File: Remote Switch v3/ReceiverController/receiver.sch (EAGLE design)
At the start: 40 parts, among them IC1 LNK304, IC2 MCP1703CB, IC3 STM8L101F2, J1 POWER_CONN_4, T1 BT136

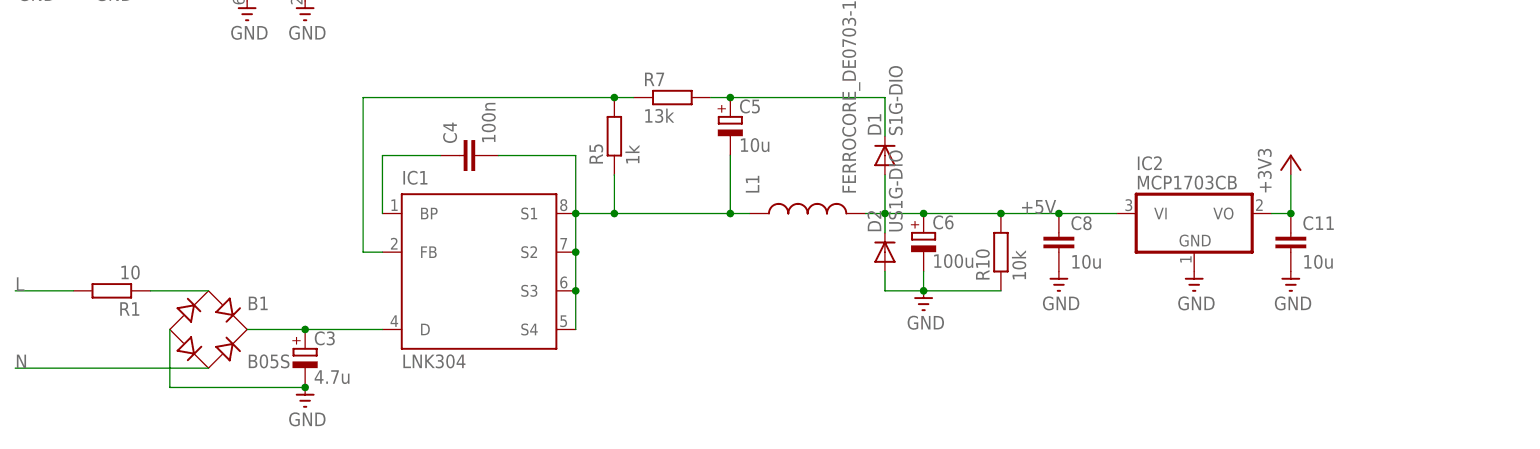
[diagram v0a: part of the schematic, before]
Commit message: PCB work
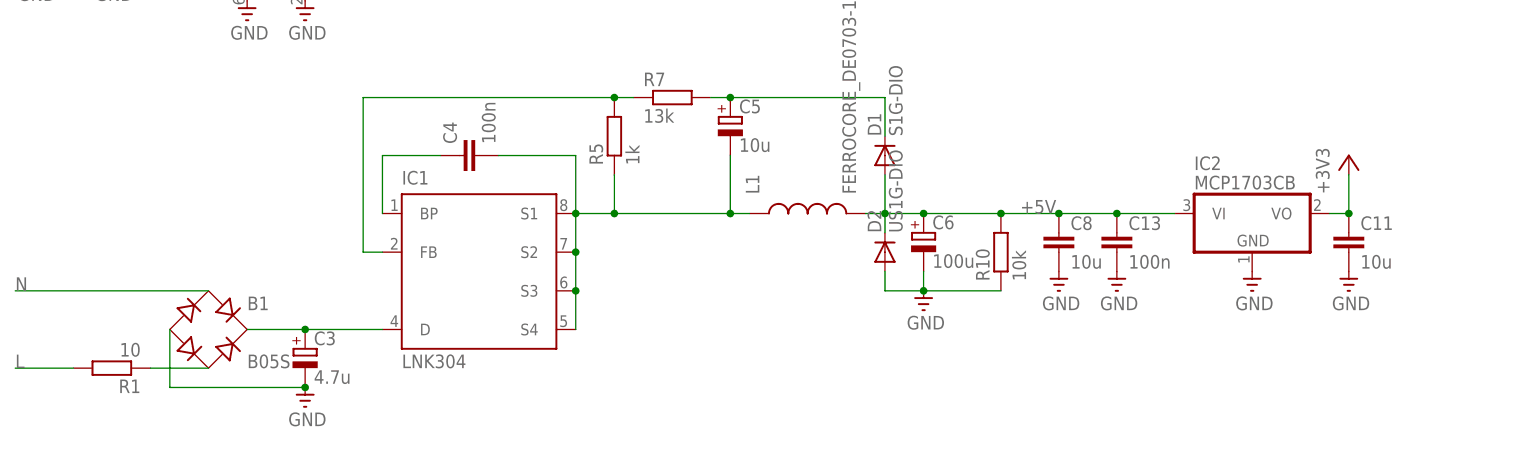
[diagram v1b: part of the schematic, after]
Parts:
- added C13: 100n, resistor:C-EUC0603K
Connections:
- removed net N$19: B1.AC1, R1.1
- new net N$10: B1.AC2, R1.1
- net +5V: now also C13.1
- net GND: now also C13.2
- net N: now also B1.AC1; no longer B1.AC2
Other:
- moved on the sheet: C11, IC2, R1
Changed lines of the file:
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@@
 <part name="GND1" library="supply" deviceset="GND" device=""/>
 <part name="R12" library="resistor" deviceset="R-EU_" device="R0603" value="47"/>
+<part name="C13" library="resistor" deviceset="C-EU" device="C0603K" value="100n"/>
+<part name="GND17" library="supply" deviceset="GND" device=""/>
 </parts>
 <sheets>
@@
 <instance part="GND15" gate="1" x="182.88" y="157.48" rot="R270"/>
 <instance part="LED1" gate="G$1" x="53.34" y="162.56" rot="R270"/>
-<instance part="R1" gate="G$1" x="25.4" y="43.18" rot="R180"/>
+<instance part="R1" gate="G$1" x="25.4" y="33.02" rot="R180"/>
 <instance part="C10" gate="G$1" x="160.02" y="142.24"/>
 <instance part="IC1" gate="G$1" x="73.66" y="45.72"/>
 <instance part="GND8" gate="1" x="132.08" y="40.64"/>
 <instance part="GND5" gate="1" x="50.8" y="27.94"/>
-<instance part="+3V34" gate="G$1" x="180.34" y="60.96"/>
+<instance part="+3V34" gate="G$1" x="187.96" y="60.96"/>
 <instance part="D2" gate="G$1" x="127" y="48.26" rot="R90"/>
 <instance part="L1" gate="G$1" x="116.84" y="53.34" rot="R90"/>
@@
 <instance part="R3" gate="G$1" x="63.5" y="134.62"/>
 <instance part="GND6" gate="1" x="66.04" y="121.92"/>
-<instance part="IC2" gate="G$1" x="167.64" y="53.34"/>
-<instance part="C11" gate="G$1" x="180.34" y="50.8"/>
-<instance part="GND14" gate="1" x="180.34" y="43.18"/>
+<instance part="IC2" gate="G$1" x="175.26" y="53.34"/>
+<instance part="C11" gate="G$1" x="187.96" y="50.8"/>
+<instance part="GND14" gate="1" x="187.96" y="43.18"/>
 <instance part="C8" gate="G$1" x="149.86" y="50.8"/>
-<instance part="GND13" gate="1" x="167.64" y="43.18"/>
+<instance part="GND13" gate="1" x="175.26" y="43.18"/>
 <instance part="GND10" gate="1" x="149.86" y="43.18"/>
 <instance part="RF1" gate="G$1" x="45.72" y="93.98"/>
@@
 <instance part="GND1" gate="1" x="15.24" y="83.82"/>
 <instance part="R12" gate="G$1" x="220.98" y="109.22"/>
+<instance part="C13" gate="G$1" x="157.48" y="50.8"/>
+<instance part="GND17" gate="1" x="157.48" y="43.18"/>
 </instances>
 <busses>
@@
 <junction x="238.76" y="134.62"/>
 <junction x="241.3" y="134.62"/>
+</segment>
+<segment>
+<pinref part="C13" gate="G$1" pin="2"/>
+<pinref part="GND17" gate="1" pin="GND"/>
 </segment>
 </net>
@@
 <pinref part="IC2" gate="G$1" pin="VO"/>
 <pinref part="C11" gate="G$1" pin="1"/>
-<wire x1="177.8" y1="53.34" x2="180.34" y2="53.34" width="0.1524" layer="91"/>
+<wire x1="185.42" y1="53.34" x2="187.96" y2="53.34" width="0.1524" layer="91"/>
 <pinref part="+3V34" gate="G$1" pin="+3V3"/>
-<wire x1="180.34" y1="53.34" x2="180.34" y2="58.42" width="0.1524" layer="91"/>
-<junction x="180.34" y="53.34"/>
+<wire x1="187.96" y1="53.34" x2="187.96" y2="58.42" width="0.1524" layer="91"/>
+<junction x="187.96" y="53.34"/>
 </segment>
 <segment>
@@
 </segment>
 <segment>
-<wire x1="38.1" y1="33.02" x2="12.7" y2="33.02" width="0.1524" layer="91"/>
-<label x="12.7" y="33.02" size="1.778" layer="95"/>
-<pinref part="B1" gate="G$1" pin="AC2"/>
+<pinref part="B1" gate="G$1" pin="AC1"/>
+<wire x1="38.1" y1="43.18" x2="12.7" y2="43.18" width="0.1524" layer="91"/>
+<label x="12.7" y="43.18" size="1.778" layer="95"/>
 </segment>
 </net>
@@
 </segment>
 </net>
-<net name="N$19" class="0">
-<segment>
-<pinref part="R1" gate="G$1" pin="1"/>
-<pinref part="B1" gate="G$1" pin="AC1"/>
-<wire x1="30.48" y1="43.18" x2="38.1" y2="43.18" width="0.1524" layer="91"/>
-</segment>
-</net>
 <net name="L" class="0">
 <segment>
@@
 <segment>
 <pinref part="R1" gate="G$1" pin="2"/>
-<wire x1="20.32" y1="43.18" x2="12.7" y2="43.18" width="0.1524" layer="91"/>
-<label x="12.7" y="43.18" size="1.778" layer="95"/>
+<wire x1="20.32" y1="33.02" x2="12.7" y2="33.02" width="0.1524" layer="91"/>
+<label x="12.7" y="33.02" size="1.778" layer="95"/>
 </segment>
 <segment>
@@
 <junction x="132.08" y="53.34"/>
 <pinref part="IC2" gate="G$1" pin="VI"/>
-<wire x1="157.48" y1="53.34" x2="149.86" y2="53.34" width="0.1524" layer="91"/>
+<wire x1="165.1" y1="53.34" x2="157.48" y2="53.34" width="0.1524" layer="91"/>
 <junction x="142.24" y="53.34"/>
 <pinref part="C8" gate="G$1" pin="1"/>
+<wire x1="157.48" y1="53.34" x2="149.86" y2="53.34" width="0.1524" layer="91"/>
 <wire x1="149.86" y1="53.34" x2="142.24" y2="53.34" width="0.1524" layer="91"/>
 <junction x="149.86" y="53.34"/>
 <label x="144.78" y="53.34" size="1.778" layer="95"/>
+<pinref part="C13" gate="G$1" pin="1"/>
+<junction x="157.48" y="53.34"/>
 </segment>
 </net>
@@
 </segment>
 </net>
+<net name="N$10" class="0">
+<segment>
+<pinref part="R1" gate="G$1" pin="1"/>
+<pinref part="B1" gate="G$1" pin="AC2"/>
+<wire x1="30.48" y1="33.02" x2="38.1" y2="33.02" width="0.1524" layer="91"/>
+</segment>
+</net>
